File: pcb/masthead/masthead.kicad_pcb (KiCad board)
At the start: 2 copper layers, 48.6 x 56.5 mm, 11 parts, among them J1 Screw_Terminal_01x01, J2 Screw_Terminal_01x01, SW1 TILT, U1 TSR_1-2450, U2 WeMos_mini, U3 BMP581

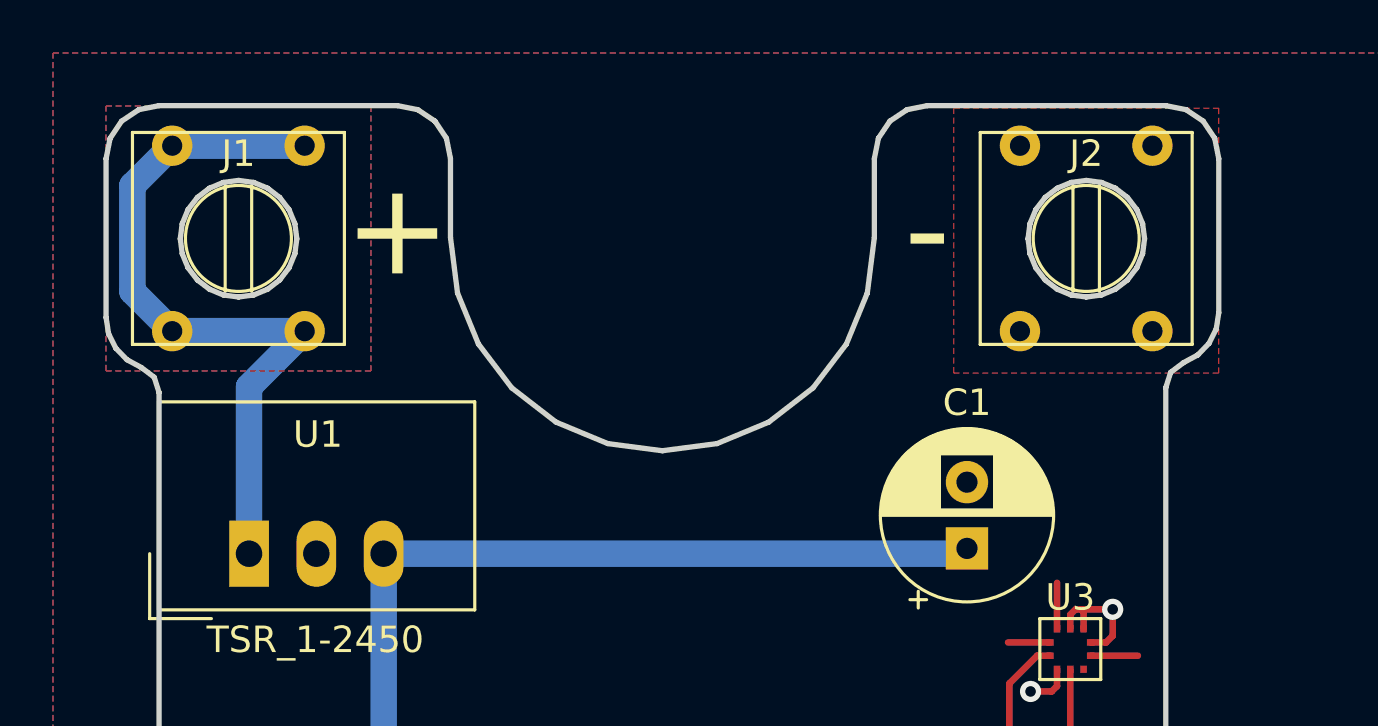
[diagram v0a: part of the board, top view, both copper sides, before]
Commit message: PCB tweak
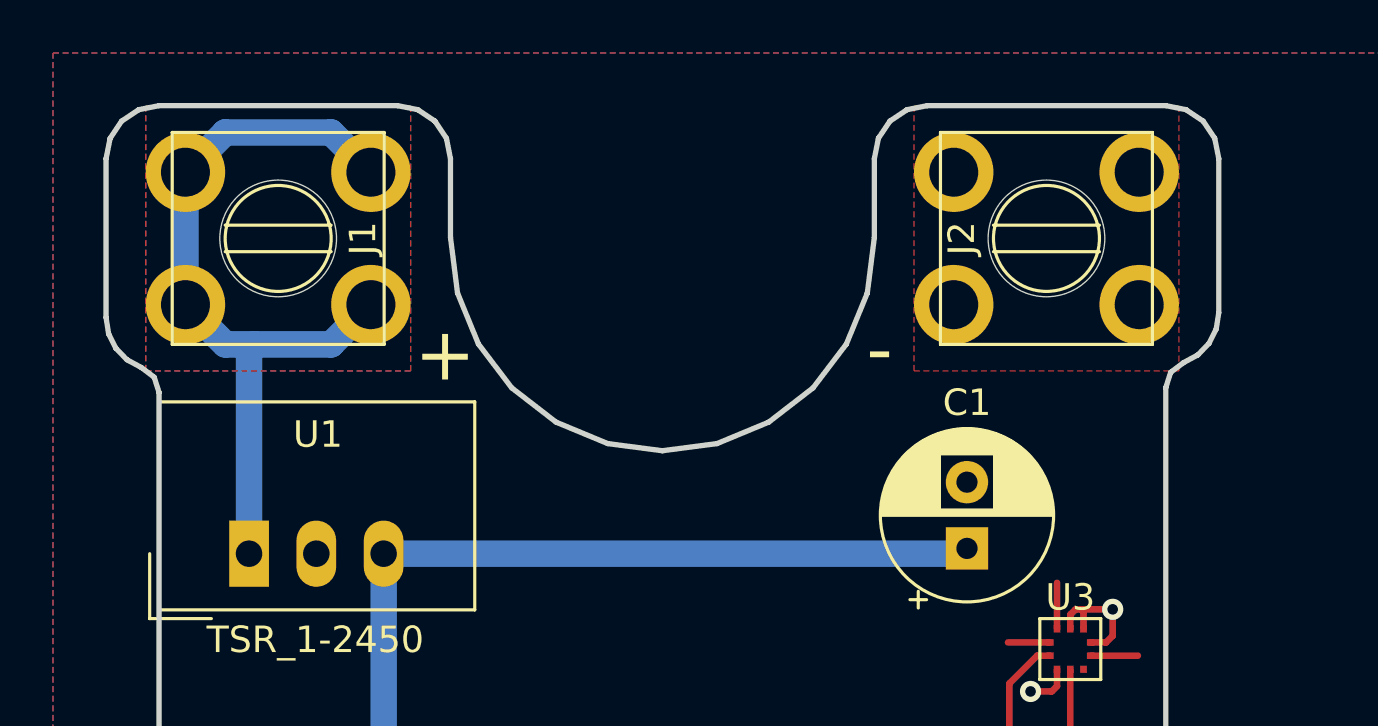
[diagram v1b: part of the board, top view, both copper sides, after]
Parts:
- moved J1 1.50 mm to (-14.5, 0.00), turned to 0 degrees
- moved J2 1.50 mm to (14.5, 0.00), turned to 180 degrees
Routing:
- net Net-(J1-Pad1): track 27.5 -> 29.5 mm
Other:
- outline, holes or cut-outs redrawn
